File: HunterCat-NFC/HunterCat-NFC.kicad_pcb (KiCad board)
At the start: 2 copper layers, 108 x 53.8 mm, 75 parts, among them J1 Battery, J2 Breakout Conn, P1 USB_C_Plug_USB2.0, U1 ATSAMD21E18A, U2 PN7150B0HN_C11002E-PN7150B0HN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, U3 MCP73831-3-OT, U4 AP2112K-3.3, U5 W25Q32JVSS, Y1 27.12Mhz

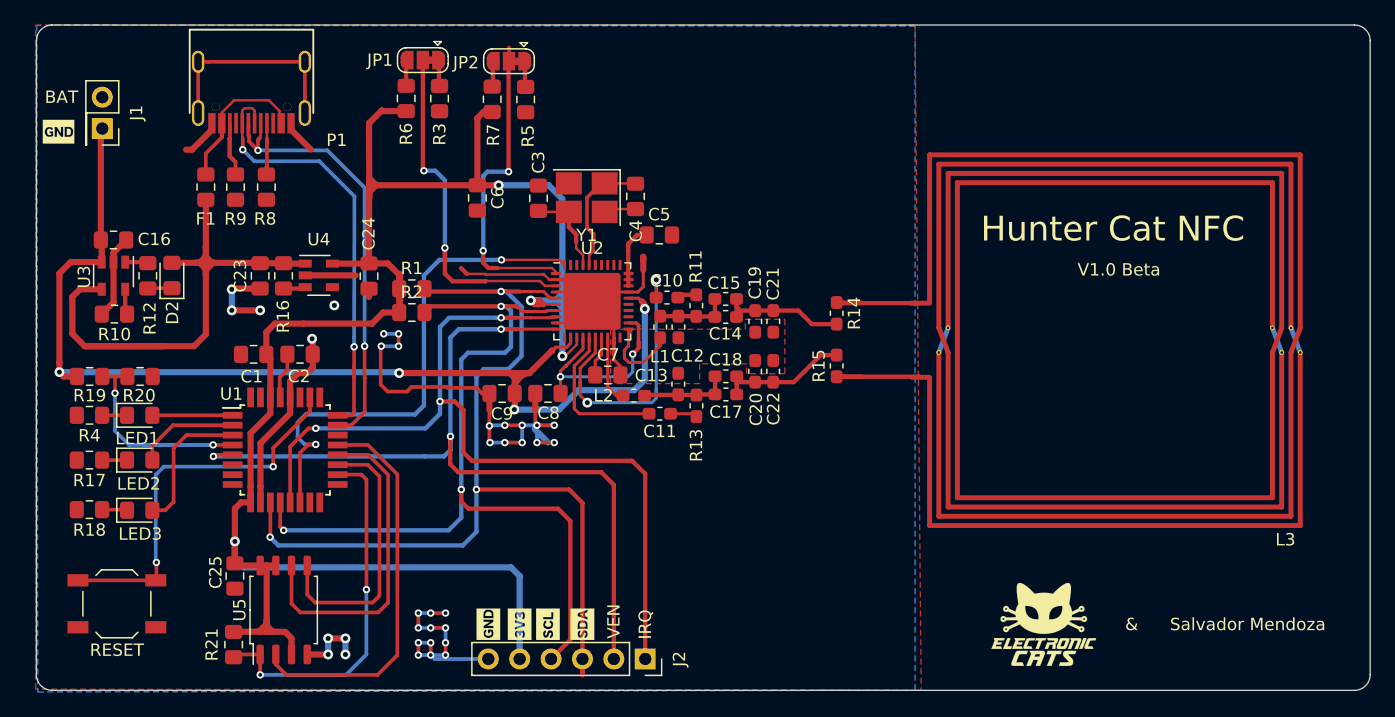
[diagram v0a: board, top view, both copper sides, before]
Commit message: Reduction
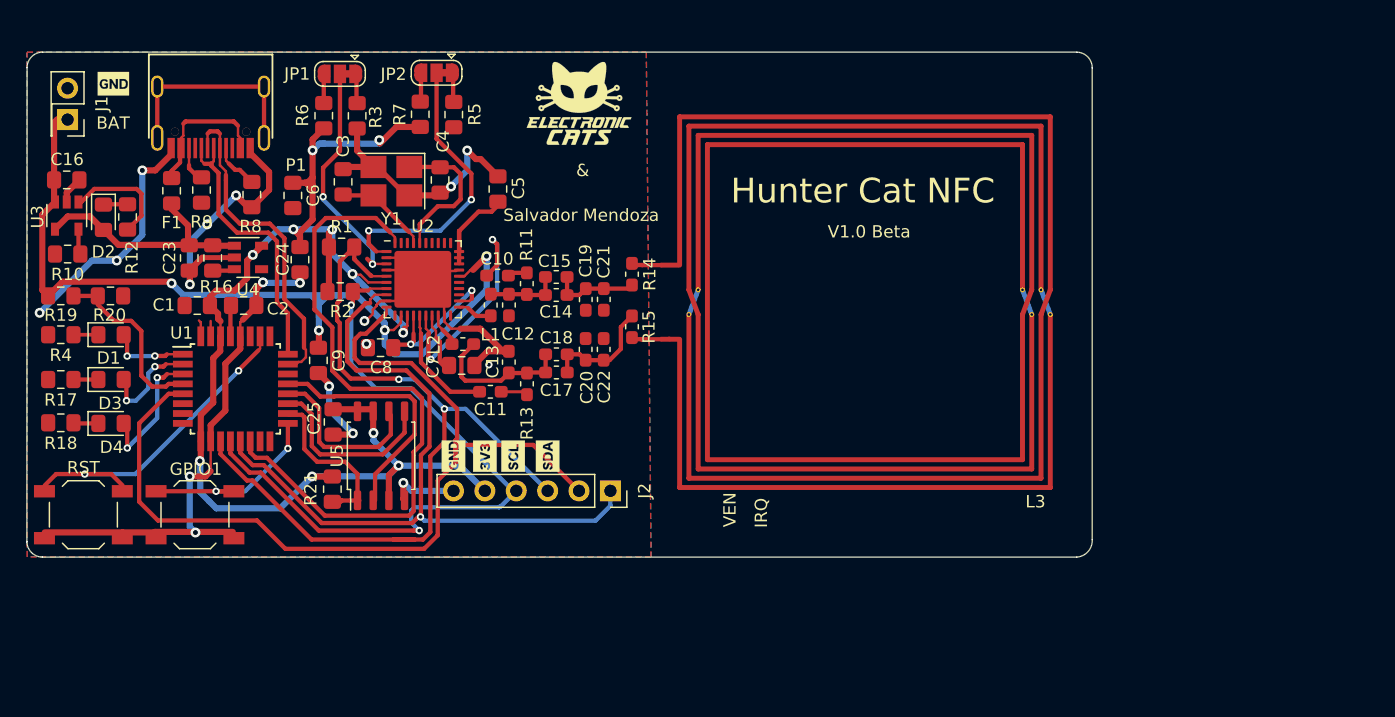
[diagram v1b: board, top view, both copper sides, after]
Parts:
- removed RESET: RESET, Button_Switch_SMD:SW_SPST_TL3342
- added GPIO1: RESET, Button_Switch_SMD:SW_SPST_TL3342, F.Cu at (116.7, 113.0)
- added RST: RESET, Button_Switch_SMD:SW_SPST_TL3342, F.Cu at (107.7, 113.0)
- U5: value W25Q32JVSS -> GD25Q16CSIGR
- moved G*** 56.5 mm to (147.8, 79.8)
- moved REF** 20.6 mm to (171.3, 98.0)
- moved L3 20.5 mm to (170.9, 95.8)
- moved R14 16.9 mm to (152.1, 93.6)
- moved R15 16.9 mm to (152.1, 97.8)
- moved C3 15.9 mm to (128.7, 86.1)
- moved C4 15.9 mm to (136.6, 85.9)
- moved Y1 15.9 mm to (132.6, 86.0)
- moved C9 15.1 mm to (126.7, 100.5), turned to 270 degrees
- moved C6 14.9 mm to (124.6, 87.2)
- moved R21 14.9 mm to (127.8, 111.0)
- moved C25 14.8 mm to (127.9, 105.5)
- moved U5 14.8 mm to (131.8, 108.3)
- moved L2 14.5 mm to (138.4, 99.2)
- moved C8 14.0 mm to (131.7, 99.5)
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- renumbered LED1 to D1, LED2 to D3, LED3 to D4
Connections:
- U1 pad 17: Net-(U1-Pad17) -> /GPIO
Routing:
- net +3V3: track 155.4 -> 115.9 mm, vias 4 -> 11
- net VBUS: track 50.6 -> 19.9 mm
- net +BATT: track 92.3 -> 73.1 mm
- net /GPIO: track 0.00 -> 17.9 mm, vias 0 -> 2
- net /CS: track 30.6 -> 13.1 mm, vias 2 -> 0
- net /SCL: track 71.6 -> 56.3 mm, vias 3 -> 2
- net /D+: track 35.9 -> 22.8 mm, vias 2 -> 0
- net /CLK: track 41.9 -> 54.0 mm, vias 2 -> 0
- net /MISO: track 32.1 -> 20.2 mm
- net GND: track 141.1 -> 153.0 mm, vias 35 -> 17
- net /SCK: track 26.6 -> 15.3 mm
- net /ADR1: track 30.6 -> 19.6 mm
- net /SDA: track 79.3 -> 69.0 mm, vias 3 -> 2
- net /IRQ: track 70.5 -> 61.1 mm, vias 3 -> 1
- net /D-: track 35.7 -> 26.8 mm, vias 2 -> 0
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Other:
- board size 108 x 53.8 mm -> 86.2 x 40.9 mm
- net class Source removed
- net class sa added: clearance 0.2, trace_width 0.2, via_dia 0.4, via_drill 0.3
- net class source added: clearance 0.2, trace_width 0.5, via_dia 0.8, via_drill 0.4
